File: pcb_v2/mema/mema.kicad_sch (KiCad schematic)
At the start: 21 parts, among them J1 bus_mem_1, J2 bus_mem_2, J3 cartridge, U1 CY62256-70PC, U2 CY62256-70PC, U3 74LS283, U4 74LS00, U5 74LS32, U7 74LS138

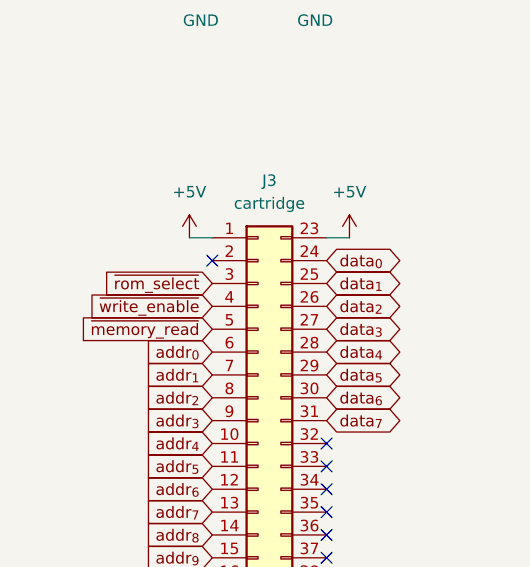
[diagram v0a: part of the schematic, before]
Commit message: roteamento com problemas; refazer
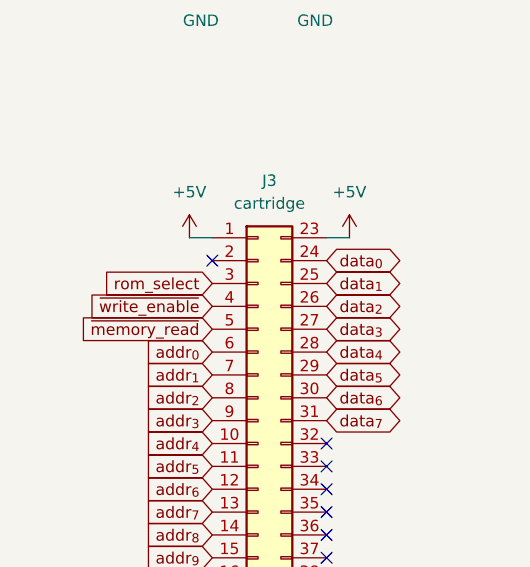
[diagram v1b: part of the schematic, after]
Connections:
- net ~{rom_select} is gone; now on net rom_select: J3.3 (Pin_3)
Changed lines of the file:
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@@
 		)
 	)
-	(global_label "~{rom_select}"
+	(global_label "rom_select"
 		(shape input)
 		(at 30.48 87.63 180)

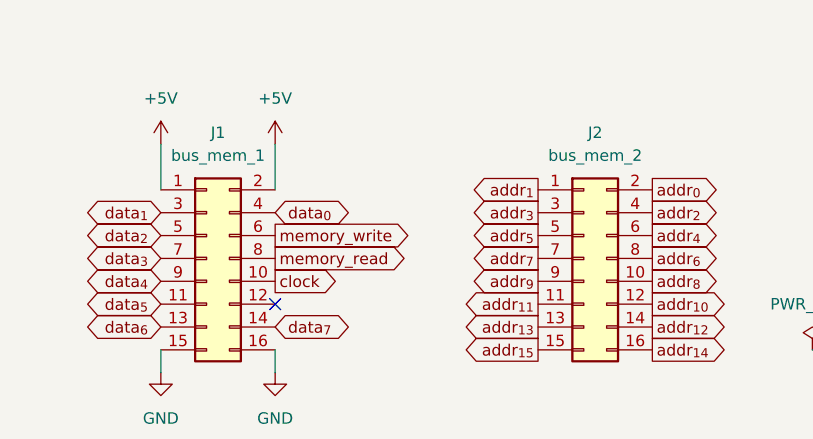
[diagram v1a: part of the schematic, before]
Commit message: concluído o roteamento
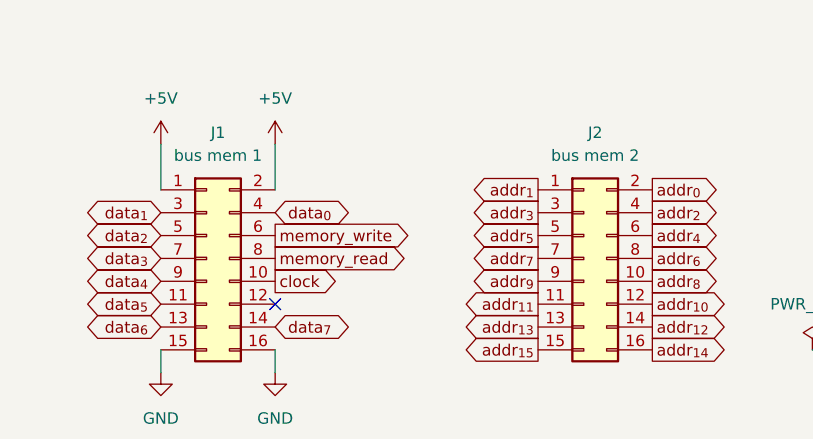
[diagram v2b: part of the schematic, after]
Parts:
- J1: value bus_mem_1 -> bus mem 1
- J2: value bus_mem_2 -> bus mem 2
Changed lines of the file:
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@@
 			)
 		)
-		(property "Value" "bus_mem_1"
+		(property "Value" "bus mem 1"
 			(at 35.56 29.21 0)
 			(effects
@@
 			)
 		)
-		(property "Value" "bus_mem_2"
+		(property "Value" "bus mem 2"
 			(at 77.47 29.21 0)
 			(effects

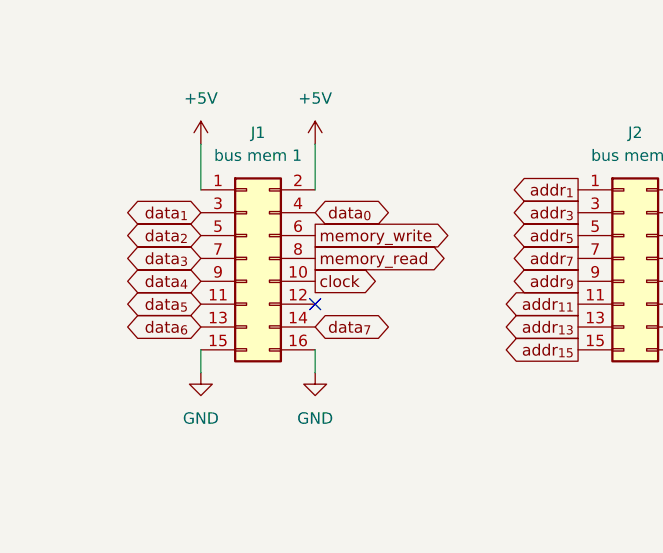
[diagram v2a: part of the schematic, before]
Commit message: experimentação com opcodes
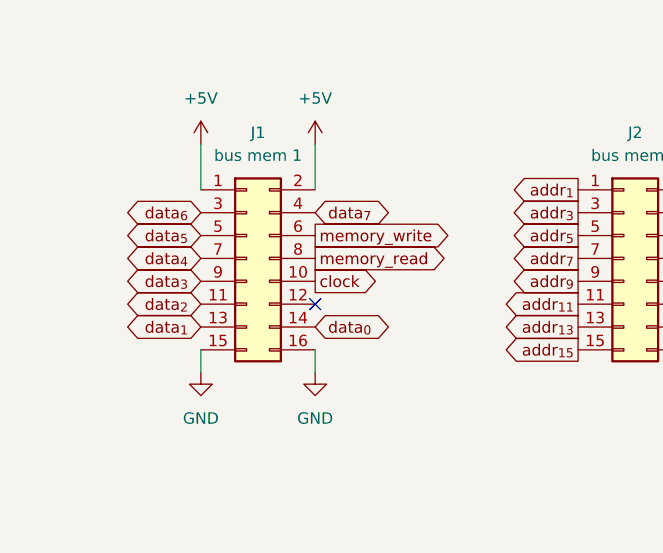
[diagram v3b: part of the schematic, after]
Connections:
- net data_{0}: now also J1.14 (Pin_14); no longer J1.4 (Pin_4)
- net data_{1}: now also J1.13 (Pin_13); no longer J1.3 (Pin_3)
- net data_{2}: now also J1.11 (Pin_11); no longer J1.5 (Pin_5)
- net data_{3}: now also J1.9 (Pin_9); no longer J1.7 (Pin_7)
- net data_{4}: now also J1.7 (Pin_7); no longer J1.9 (Pin_9)
- net data_{5}: now also J1.5 (Pin_5); no longer J1.11 (Pin_11)
- net data_{6}: now also J1.3 (Pin_3); no longer J1.13 (Pin_13)
- net data_{7}: now also J1.4 (Pin_4); no longer J1.14 (Pin_14)
